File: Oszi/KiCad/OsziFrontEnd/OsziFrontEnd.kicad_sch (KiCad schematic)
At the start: 0 parts

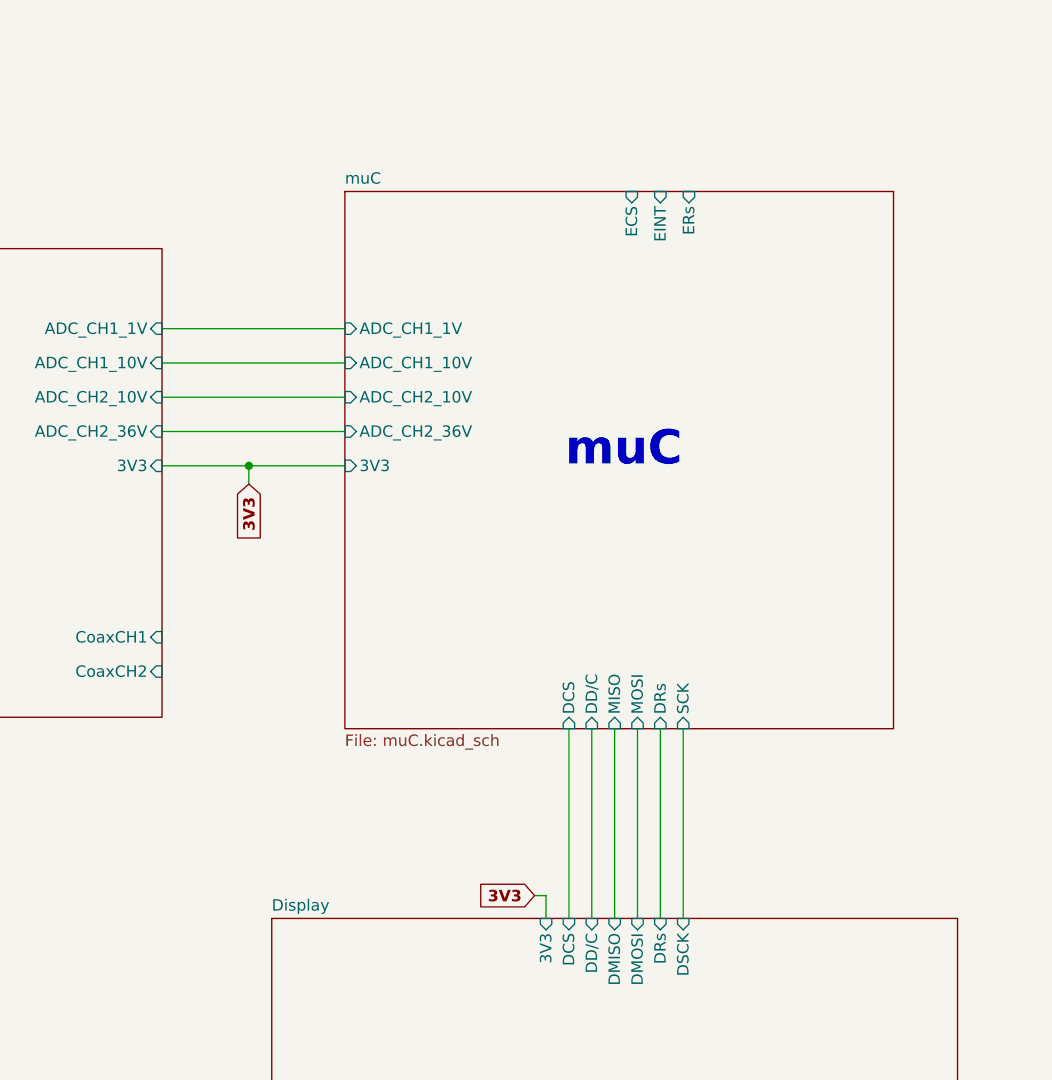
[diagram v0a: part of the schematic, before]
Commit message: jetzt git
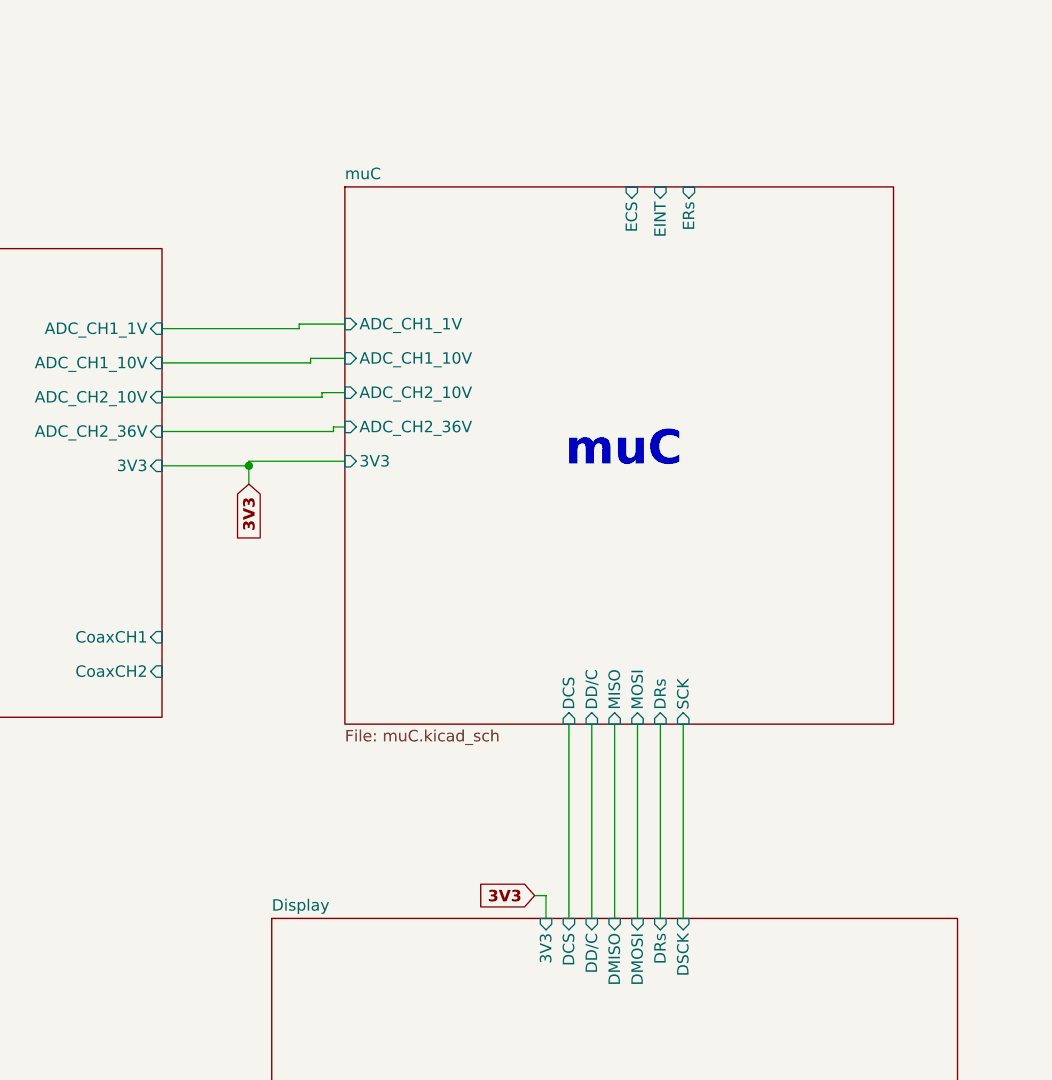
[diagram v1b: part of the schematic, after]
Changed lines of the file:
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@@
+	(wire
+		(pts
+			(xy 262.128 124.46) (xy 262.128 124.968)
+		)
+		(stroke
+			(width 0)
+			(type default)
+		)
+	)
+	(wire
+		(pts
+			(xy 260.858 121.158) (xy 244.348 121.158)
+		)
+		(stroke
+			(width 0)
+			(type default)
+		)
+	)
 	(wire
 		(pts
@@
 	(wire
 		(pts
-			(xy 302.26 161.798) (xy 302.26 182.88)
-		)
-		(stroke
-			(width 0)
-			(type default)
-		)
-	)
-	(wire
-		(pts
-			(xy 254 132.588) (xy 264.668 132.588)
-		)
-		(stroke
-			(width 0)
-			(type default)
-		)
-	)
-	(wire
-		(pts
-			(xy 289.56 161.798) (xy 289.56 182.88)
+			(xy 302.26 161.29) (xy 302.26 182.88)
+		)
+		(stroke
+			(width 0)
+			(type default)
+		)
+	)
+	(wire
+		(pts
+			(xy 254 132.08) (xy 264.668 132.08)
+		)
+		(stroke
+			(width 0)
+			(type default)
+		)
+	)
+	(wire
+		(pts
+			(xy 259.588 117.348) (xy 244.348 117.348)
+		)
+		(stroke
+			(width 0)
+			(type default)
+		)
+	)
+	(wire
+		(pts
+			(xy 260.858 120.65) (xy 260.858 121.158)
+		)
+		(stroke
+			(width 0)
+			(type default)
+		)
+	)
+	(wire
+		(pts
+			(xy 289.56 161.29) (xy 289.56 182.88)
+		)
+		(stroke
+			(width 0)
+			(type default)
+		)
+	)
+	(wire
+		(pts
+			(xy 259.588 116.84) (xy 259.588 117.348)
 		)
 		(stroke
@@
 	(wire
 		(pts
-			(xy 292.1 161.798) (xy 292.1 182.88)
-		)
-		(stroke
-			(width 0)
-			(type default)
-		)
-	)
-	(wire
-		(pts
-			(xy 294.64 161.798) (xy 294.64 182.88)
-		)
-		(stroke
-			(width 0)
-			(type default)
-		)
-	)
-	(wire
-		(pts
-			(xy 244.348 128.778) (xy 264.668 128.778)
-		)
-		(stroke
-			(width 0)
-			(type default)
-		)
-	)
-	(wire
-		(pts
-			(xy 244.348 117.348) (xy 264.668 117.348)
-		)
-		(stroke
-			(width 0)
-			(type default)
-		)
-	)
-	(wire
-		(pts
-			(xy 297.18 161.798) (xy 297.18 182.88)
-		)
-		(stroke
-			(width 0)
-			(type default)
-		)
-	)
-	(wire
-		(pts
-			(xy 244.348 121.158) (xy 264.668 121.158)
-		)
-		(stroke
-			(width 0)
-			(type default)
-		)
-	)
-	(wire
-		(pts
-			(xy 244.348 124.968) (xy 264.668 124.968)
+			(xy 292.1 161.29) (xy 292.1 182.88)
+		)
+		(stroke
+			(width 0)
+			(type default)
+		)
+	)
+	(wire
+		(pts
+			(xy 263.398 128.27) (xy 263.398 128.778)
+		)
+		(stroke
+			(width 0)
+			(type default)
+		)
+	)
+	(wire
+		(pts
+			(xy 294.64 161.29) (xy 294.64 182.88)
+		)
+		(stroke
+			(width 0)
+			(type default)
+		)
+	)
+	(wire
+		(pts
+			(xy 263.398 128.27) (xy 264.668 128.27)
+		)
+		(stroke
+			(width 0)
+			(type default)
+		)
+	)
+	(wire
+		(pts
+			(xy 259.588 116.84) (xy 264.668 116.84)
+		)
+		(stroke
+			(width 0)
+			(type default)
+		)
+	)
+	(wire
+		(pts
+			(xy 263.398 128.778) (xy 244.348 128.778)
+		)
+		(stroke
+			(width 0)
+			(type default)
+		)
+	)
+	(wire
+		(pts
+			(xy 254 132.08) (xy 254 132.588)
+		)
+		(stroke
+			(width 0)
+			(type default)
+		)
+	)
+	(wire
+		(pts
+			(xy 297.18 161.29) (xy 297.18 182.88)
+		)
+		(stroke
+			(width 0)
+			(type default)
+		)
+	)
+	(wire
+		(pts
+			(xy 260.858 120.65) (xy 264.668 120.65)
+		)
+		(stroke
+			(width 0)
+			(type default)
+		)
+	)
+	(wire
+		(pts
+			(xy 262.128 124.46) (xy 264.668 124.46)
 		)
 		(stroke
@@
 	(wire
 		(pts
-			(xy 299.72 161.798) (xy 299.72 182.88)
+			(xy 299.72 161.29) (xy 299.72 182.88)
+		)
+		(stroke
+			(width 0)
+			(type default)
+		)
+	)
+	(wire
+		(pts
+			(xy 262.128 124.968) (xy 244.348 124.968)
 		)
 		(stroke
@@
 	)
 	(sheet
-		(at 264.668 102.108)
+		(at 264.668 101.6)
 		(size 60.96 59.69)
 		(exclude_from_sim no)
@@
 		)
 		(property "Sheetname" "muC"
-			(at 264.668 101.3964 0)
+			(at 264.668 100.8884 0)
 			(effects
 				(font
@@
 		)
 		(property "Sheetfile" "muC.kicad_sch"
-			(at 264.668 162.3826 0)
+			(at 264.668 161.8746 0)
 			(effects
 				(font
@@
 		)
 		(pin "3V3" input
-			(at 264.668 132.588 180)
+			(at 264.668 132.08 180)
 			(effects
 				(font
@@
 		)
 		(pin "ADC_CH1_1V" input
-			(at 264.668 117.348 180)
+			(at 264.668 116.84 180)
 			(effects
 				(font
@@
 		)
 		(pin "ADC_CH2_10V" input
-			(at 264.668 124.968 180)
+			(at 264.668 124.46 180)
 			(effects
 				(font
@@
 		)
 		(pin "ADC_CH2_36V" input
-			(at 264.668 128.778 180)
+			(at 264.668 128.27 180)
 			(effects
 				(font
@@
 		)
 		(pin "ADC_CH1_10V" input
-			(at 264.668 121.158 180)
+			(at 264.668 120.65 180)
 			(effects
 				(font
@@
 		)
 		(pin "DCS" input
-			(at 289.56 161.798 270)
+			(at 289.56 161.29 270)
 			(effects
 				(font
@@
 		)
 		(pin "DD{slash}C" input
-			(at 292.1 161.798 270)
+			(at 292.1 161.29 270)
 			(effects
 				(font
@@
 		)
 		(pin "DRs" input
-			(at 299.72 161.798 270)
+			(at 299.72 161.29 270)
 			(effects
 				(font
@@
 		)
 		(pin "ECS" input
-			(at 296.545 102.108 90)
+			(at 296.545 101.6 90)
 			(effects
 				(font
@@
 		)
 		(pin "EINT" input
-			(at 299.72 102.108 90)
+			(at 299.72 101.6 90)
 			(effects
 				(font
@@
 		)
 		(pin "ERs" input
-			(at 302.895 102.108 90)
+			(at 302.895 101.6 90)
 			(effects
 				(font
@@
 		)
 		(pin "MISO" input
-			(at 294.64 161.798 270)
+			(at 294.64 161.29 270)
 			(effects
 				(font
@@
 		)
 		(pin "MOSI" input
-			(at 297.18 161.798 270)
+			(at 297.18 161.29 270)
 			(effects
 				(font
@@
 		)
 		(pin "SCK" input
-			(at 302.26 161.798 270)
-			(effects
-				(font
+			(at 302.26 161.29 270)
+			(effects
+				(font
